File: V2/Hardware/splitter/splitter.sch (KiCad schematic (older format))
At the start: 17 parts, among them J0 Rpi_40Pin_F, J1 Control1_F, J2 Control2_F, J3 Control3_F, J4 Molex_PSU_F, J5 Siren, J6 USB_A_F, K0 RELRAS0515, Q0 BC548C, Q1 BD139-16

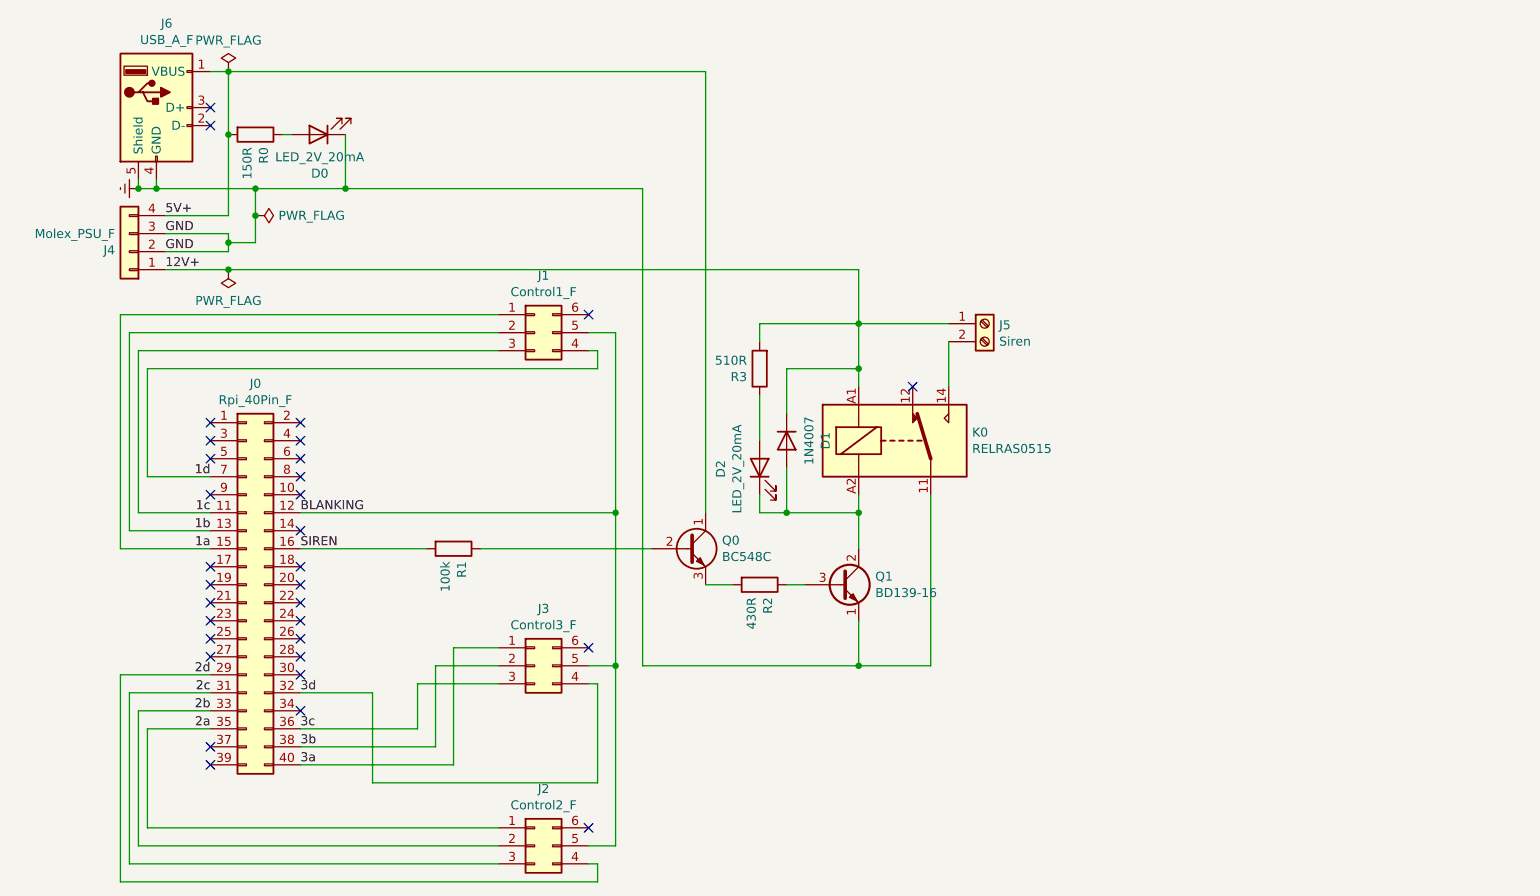
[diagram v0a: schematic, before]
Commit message: update schemas
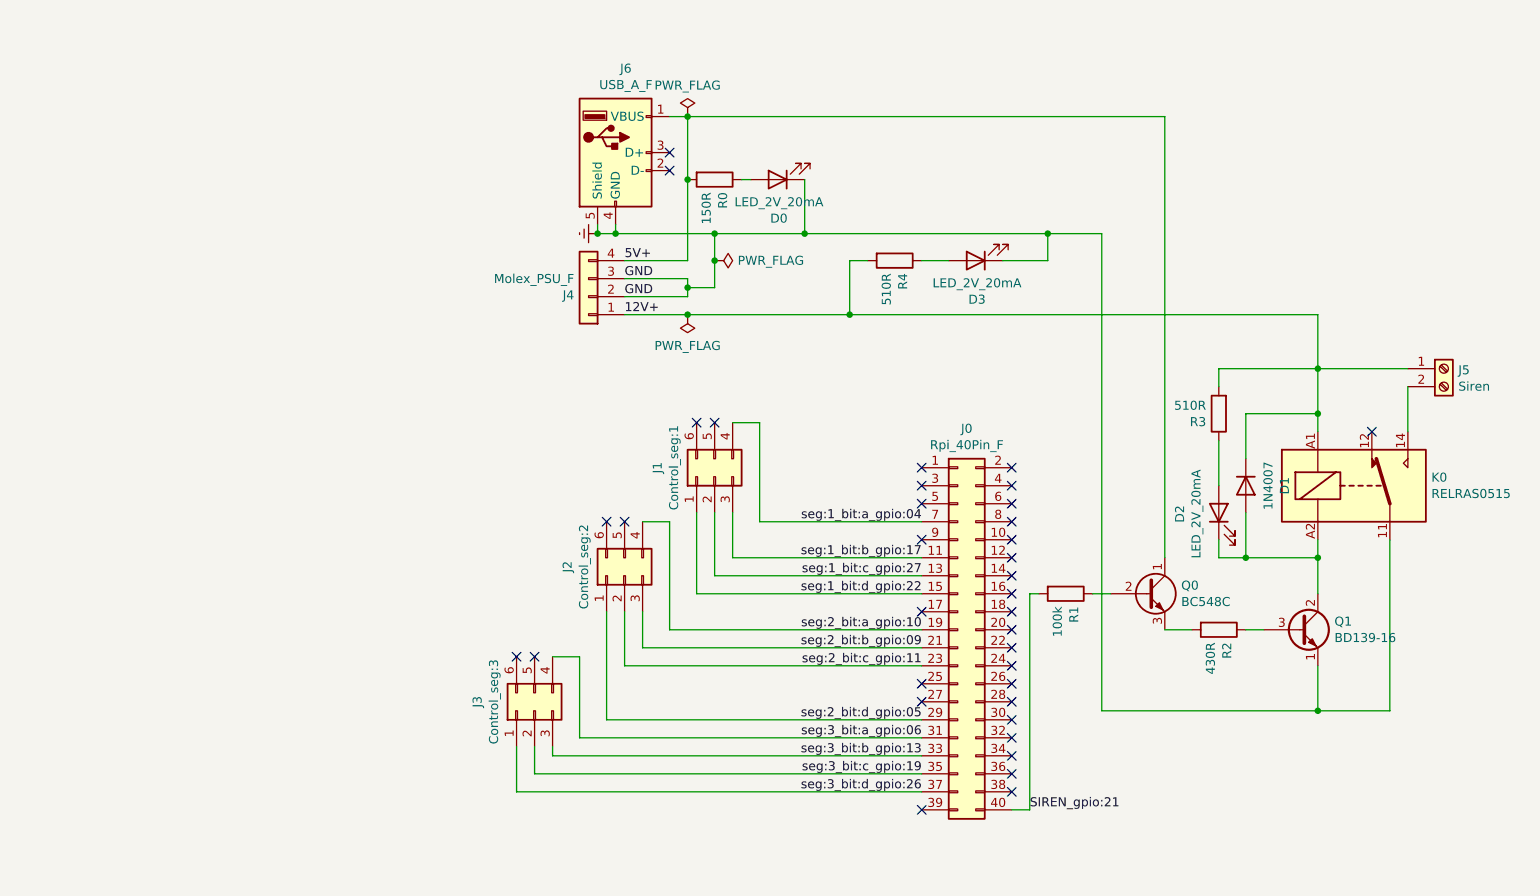
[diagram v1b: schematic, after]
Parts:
- added D3: LED_2V_20mA, LED_THT:LED_D5.0mm, symbol Device:LED
- added R4: 510R, Resistor_THT:R_Axial_DIN0207_L6.3mm_D2.5mm_P10.16mm_Horizontal, symbol Device:R
- J1: value Control1_F -> Control_seg:1
- J2: value Control2_F -> Control_seg:2
- J3: value Control3_F -> Control_seg:3
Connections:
- net 12V+: now also R4.2
- net Earth: now also D3.1 (K)
- net seg:2_bit:a_gpio:10: now reaches J0.19 (Pin_19)
- net seg:2_bit:a_gpio:10: now also J2.4 (Pin_4)
- net seg:2_bit:b_gpio:09: now reaches J0.21 (Pin_21)
- net seg:2_bit:b_gpio:09: now also J2.3 (Pin_3)
- net seg:2_bit:c_gpio:11: now reaches J0.23 (Pin_23)
- net seg:2_bit:c_gpio:11: now also J2.2 (Pin_2)
- net seg:3_bit:d_gpio:26: now reaches J0.37 (Pin_37)
- net seg:3_bit:d_gpio:26: now also J3.1 (Pin_1)
- net 1a renamed seg:1_bit:d_gpio:22
- net 1b renamed seg:1_bit:c_gpio:27
- net 1c renamed seg:1_bit:b_gpio:17
- net 1d renamed seg:1_bit:a_gpio:04
- net 2a renamed seg:2_bit:d_gpio:05
- net seg:2_bit:d_gpio:05: now also J0.29 (Pin_29); no longer J0.35 (Pin_35)
- net 2b renamed seg:3_bit:b_gpio:13
- net seg:3_bit:b_gpio:13: now also J3.3 (Pin_3); no longer J2.2 (Pin_2)
- net 2c renamed seg:3_bit:a_gpio:06
- net seg:3_bit:a_gpio:06: now also J3.4 (Pin_4); no longer J2.3 (Pin_3)
- removed net 2d: J0.29 (Pin_29), J2.4 (Pin_4)
- net 3a renamed SIREN_gpio:21
- net SIREN_gpio:21: now also R1.2; no longer J3.1 (Pin_1)
- net 3b: no longer names the net of J0.38 (Pin_38)
- net 3b: no longer J3.2 (Pin_2)
- net 3c: no longer names the net of J0.36 (Pin_36)
- net 3c: no longer J3.3 (Pin_3)
- net 3d: no longer names the net of J0.32 (Pin_32)
- net 3d: no longer J3.4 (Pin_4)
- removed net BLANKING: J0.12 (Pin_12), J1.5 (Pin_5), J2.5 (Pin_5), J3.5 (Pin_5)
- net SIREN: no longer names the net of J0.16 (Pin_16)
- net SIREN: no longer R1.2
- new net: D3.2 (A), R4.1
- new net seg:3_bit:c_gpio:19: J0.35 (Pin_35), J3.2 (Pin_2)
- no-connect marks 32 -> 36
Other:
- moved on the sheet: D0, D1, D2, J0, J1, J2, J3, J4, J5, J6, K0, Q0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
